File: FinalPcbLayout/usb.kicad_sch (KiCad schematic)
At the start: 8 parts, among them J5 USB_C_Receptacle, Q2 S8050, Q3 S8050, U2 FT231XQ

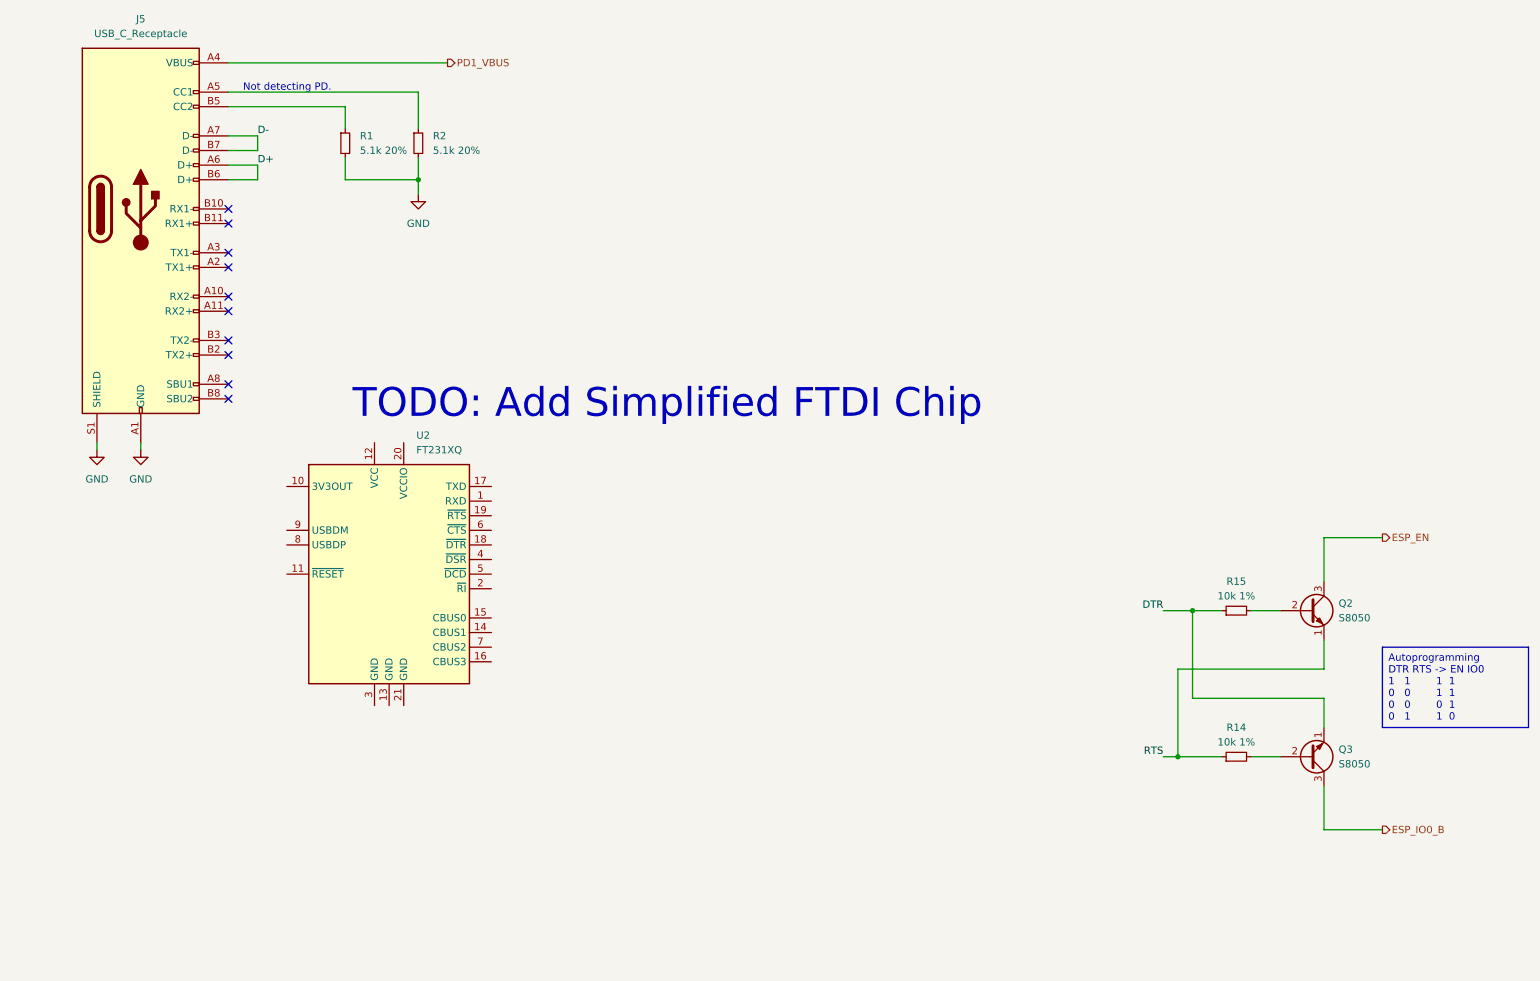
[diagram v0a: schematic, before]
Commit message: Working on USB to UART
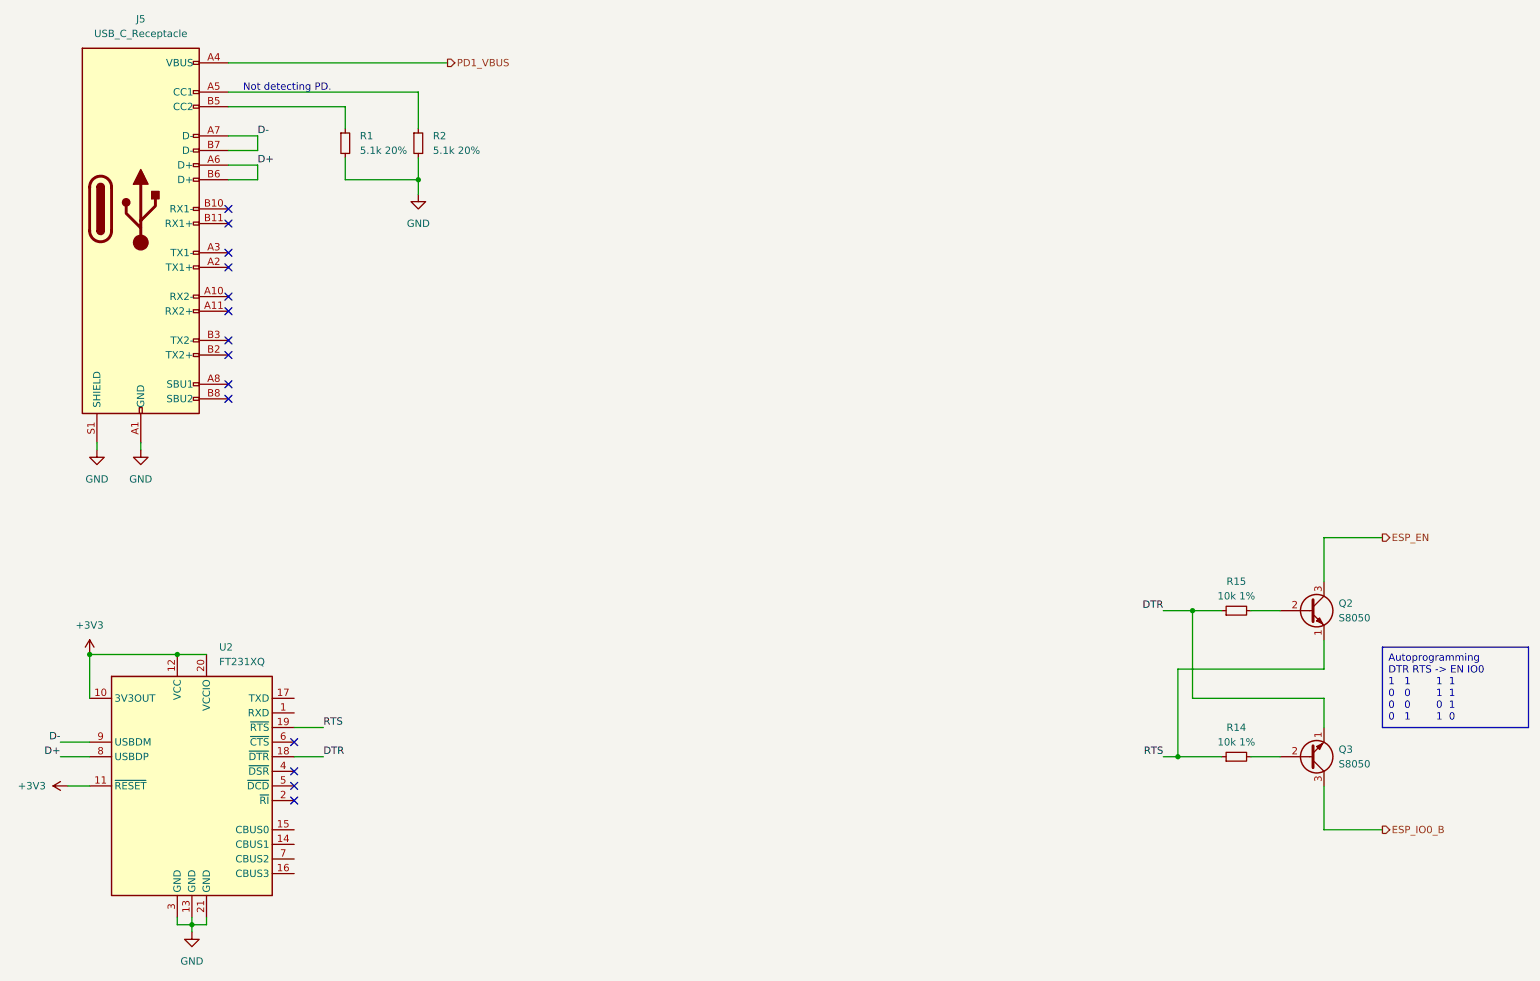
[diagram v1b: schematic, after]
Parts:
- R1, R2: footprint (none) -> Resistor_SMD:R_0603_1608Metric
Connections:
- net D+: now also U2.8 (USBDP)
- net D-: now also U2.9 (USBDM)
- net DTR: now also U2.18 (~{DTR})
- net GND: now also U2.13 (GND), U2.21 (GND), U2.3 (GND)
- net RTS: now also U2.19 (~{RTS})
- net +3V3: now reaches U2.10 (3V3OUT)
- net +3V3: now also U2.11 (~{RESET}), U2.12 (VCC), U2.20 (VCCIO)
- no-connect marks 10 -> 14
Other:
- note removed: "TODO: Add Simplified FTDI Chip"
- moved on the sheet: U2
